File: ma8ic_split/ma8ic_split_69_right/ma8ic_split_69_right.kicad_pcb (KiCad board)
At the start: 2 copper layers, 175.8 x 125.7 mm, 148 parts, among them J1 USB_C_Receptacle, J2 MJ-4PP-9, J3 I2C, J4 SPI, SW1 SW_PUSH, SW10 SW_PUSH-kbd, SW11 SW_PUSH-kbd, SW12 SW_PUSH-kbd, SW13 SW_PUSH-kbd, SW14 SW_PUSH-kbd, SW15 SW_PUSH-kbd, SW16 SW_PUSH-kbd, SW17 SW_PUSH-kbd, SW18 SW_PUSH-kbd, SW19 SW_PUSH-kbd, SW2 SW_PUSH-kbd, SW20 SW_PUSH-kbd, SW21 SW_PUSH-kbd, SW22 SW_PUSH-kbd, SW23 SW_PUSH-kbd, SW24 SW_PUSH-kbd, SW25 SW_PUSH-kbd, SW26 SW_PUSH-kbd, SW27 SW_PUSH-kbd, SW28 SW_PUSH-kbd, SW29 SW_PUSH-kbd, SW3 SW_PUSH-kbd, SW30 SW_PUSH-kbd, SW31 SW_PUSH-kbd, SW32 SW_PUSH-kbd, SW33 SW_PUSH-kbd, SW34 SW_PUSH-kbd, SW35 SW_PUSH-kbd, SW36 SW_PUSH-kbd, SW37 SW_PUSH-kbd, SW38 SW_PUSH-kbd, SW4 SW_PUSH-kbd, SW5 SW_PUSH-kbd, SW6 SW_PUSH-kbd, SW7 SW_PUSH-kbd, SW8 SW_PUSH-kbd, SW9 SW_PUSH-kbd, U1 ATMEGA32U4, X1 CSTNE16M0V530000R0

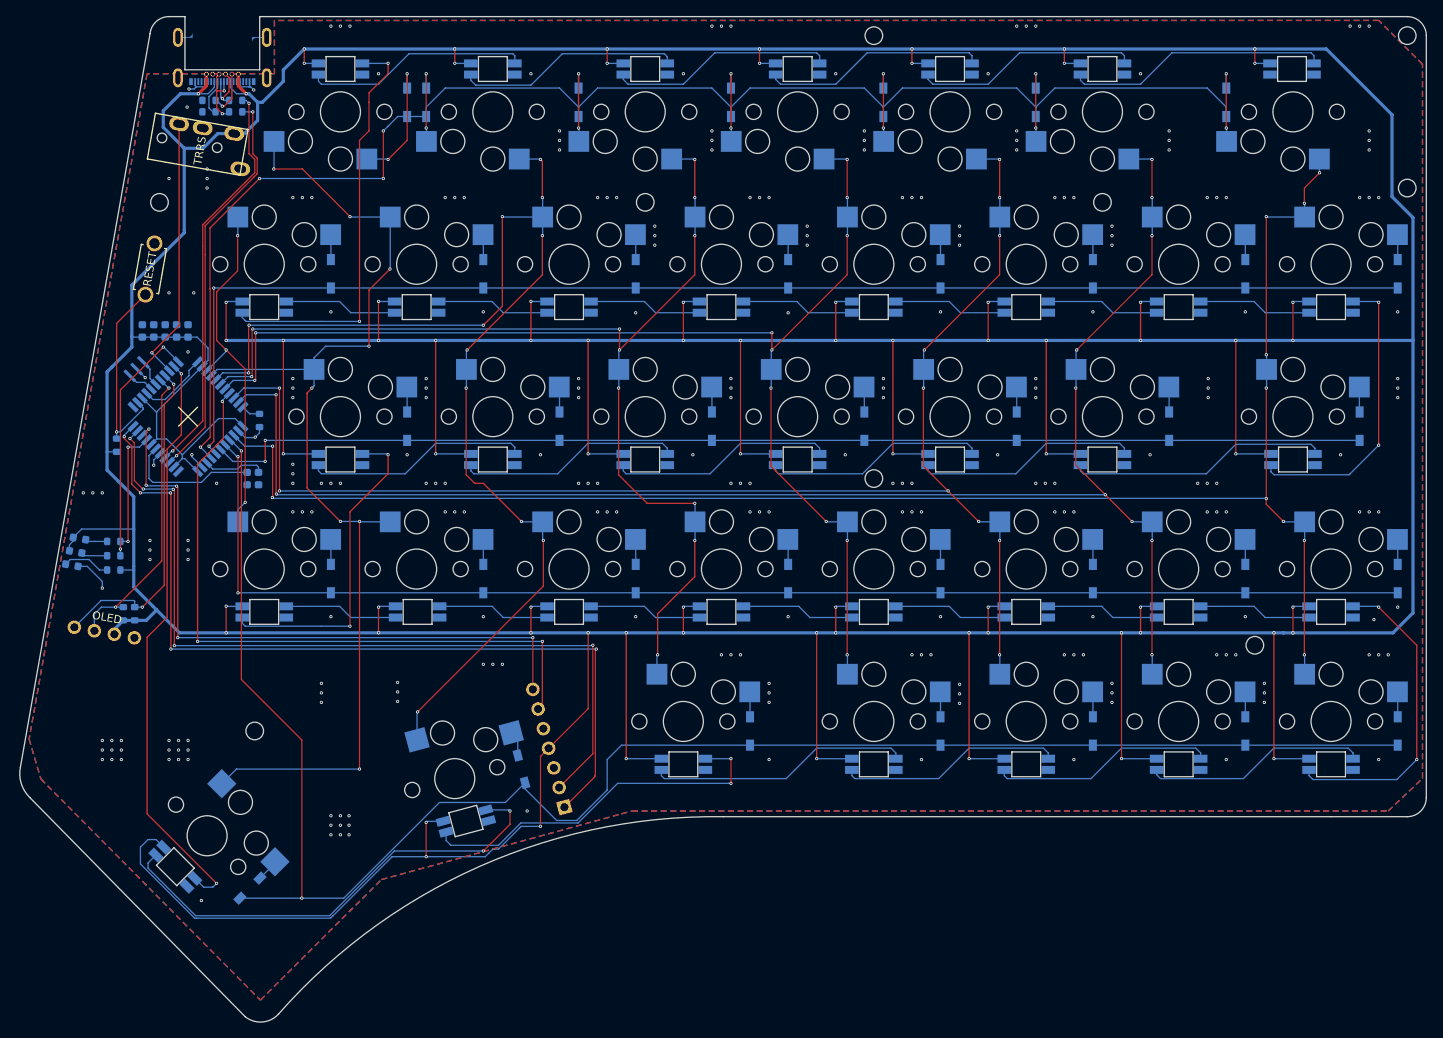
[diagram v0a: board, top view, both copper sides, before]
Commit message: update
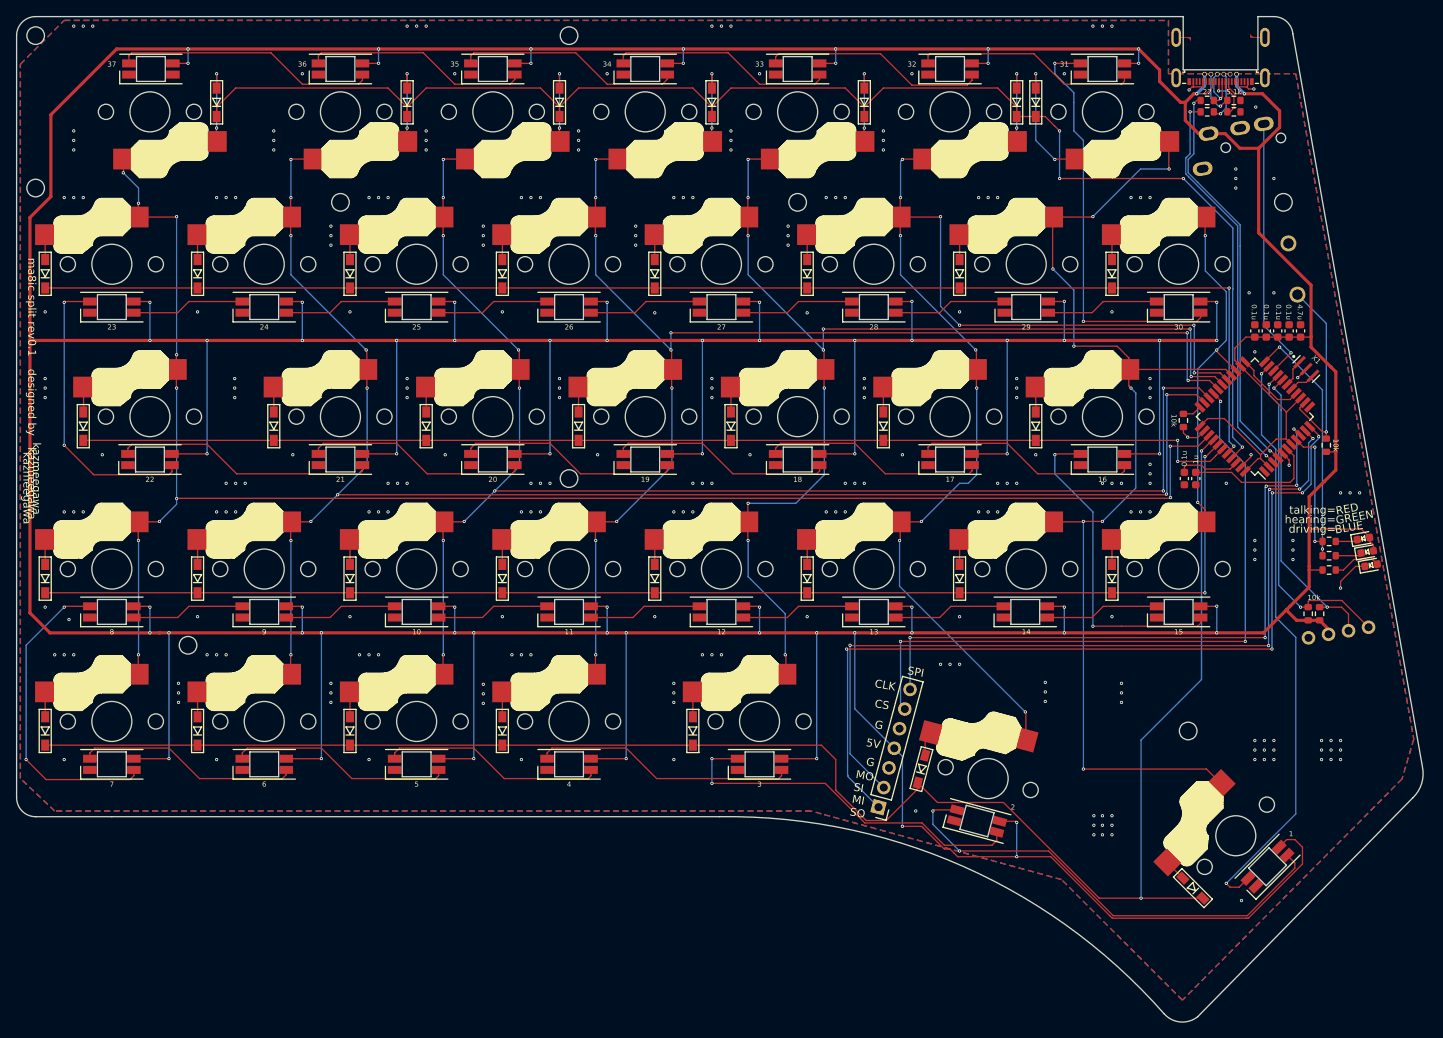
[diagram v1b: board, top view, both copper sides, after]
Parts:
- ? (x5), C1, C2, C3, C4, C5, C6, C7, D1, D10, D11, D12, D13, D14, D15, D16, D17, D18, D19, D2, D20, D21, D22, D23, D24, D25, D26, D27, D28, D29, D3, D30, D31, D32, D33, D34, D35, D36, D37, D38, D39, D4, D40, D41, D42, D43, D44, D45, D46, D47, D48, D49, D5, D50, D51, D52, D53, D54, D55, D56, D57, D58, D59, D6, D60, D61, D62, D63, D64, D65, D66, D67, D68, D69, D7, D70, D71, D72, D73, D74, D75, D76, D77, D8, D9, J1, J4, R1, R10, R11, R2, R3, R4, R5, R6, R7, R8, R9, REF** (x4), U1, X1: moved to F.Cu
- J2, J3, SW1, SW10, SW11, SW12, SW13, SW14, SW15, SW16, SW17, SW18, SW19, SW2, SW20, SW21, SW22, SW23, SW24, SW25, SW26, SW27, SW28, SW29, SW3, SW30, SW31, SW32, SW33, SW34, SW35, SW36, SW37, SW38, SW4, SW5, SW6, SW7, SW8, SW9: moved to B.Cu
- moved ? 171.5 mm to (61.9, 38.1), turned to 0 degrees
- moved ? 171.5 mm to (61.9, 57.1), turned to 0 degrees
- moved D26 169.1 mm to (63.1, 106.0)
- moved D34 169.1 mm to (63.1, 125.0)
- moved D11 169.1 mm to (63.1, 67.9)
- moved D3 162.4 mm to (228.8, 104.3), turned to 10 degrees
- moved D2 161.4 mm to (228.4, 102.6), turned to 10 degrees
- moved D1 160.5 mm to (227.9, 101.0), turned to 10 degrees
- moved D19 159.5 mm to (67.9, 86.9)
- moved J3 154.3 mm to (224.8, 112.7), turned to -170 degrees
- moved D48 152.4 mm to (71.4, 110.1), turned to 0 degrees
- moved D63 152.4 mm to (71.4, 72.0), turned to 0 degrees
- moved SW24 152.4 mm to (71.4, 104.8), turned to 0 degrees
- moved SW32 152.4 mm to (71.4, 123.8), turned to 0 degrees
- moved SW9 152.4 mm to (71.4, 66.7), turned to 0 degrees
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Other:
- outline, holes or cut-outs redrawn
